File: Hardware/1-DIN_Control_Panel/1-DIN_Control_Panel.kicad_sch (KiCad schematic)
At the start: 82 parts, among them J1 Selector Knob Connector, J2 Rotary Switch 1x7, J3 2x05 Molex Micro-Fit 3.0 43045, J4 UART Expansion, J5 SW - Aux Jump-Start, J6 SW - Battery Bypass, J7 SW - Master Power, J8 Pot/SW - Brightness, K1 FINDER-40.52, U1 CA56-12SEKWA, U2 CA56-12SEKWA, U3 LTV-847S, U4 LTV-847S, U5 MAX 6954 - SSOP, U6 MAX 6954 - SSOP, U7 LM324DR, U8 12V->5V Variable Boost Buck C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

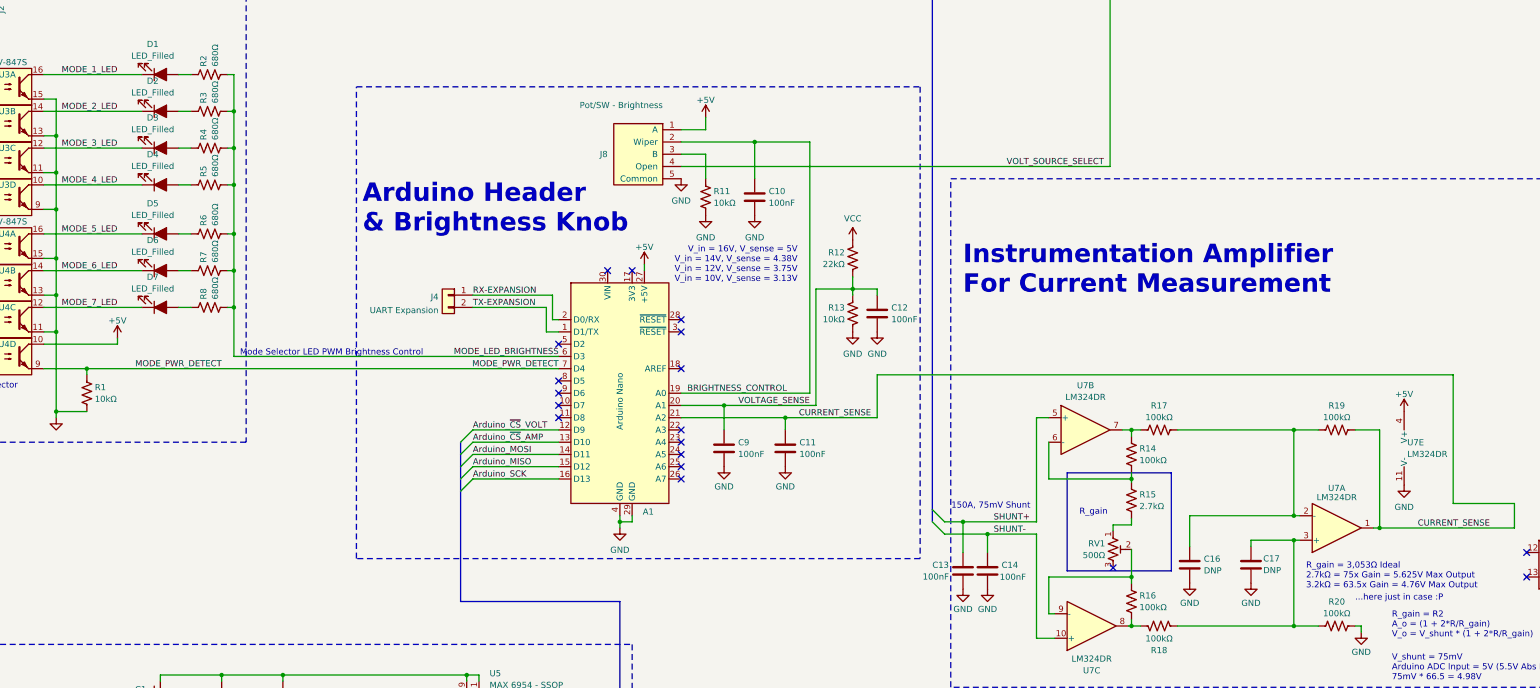
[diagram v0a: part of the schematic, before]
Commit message: Scooted some stuffs
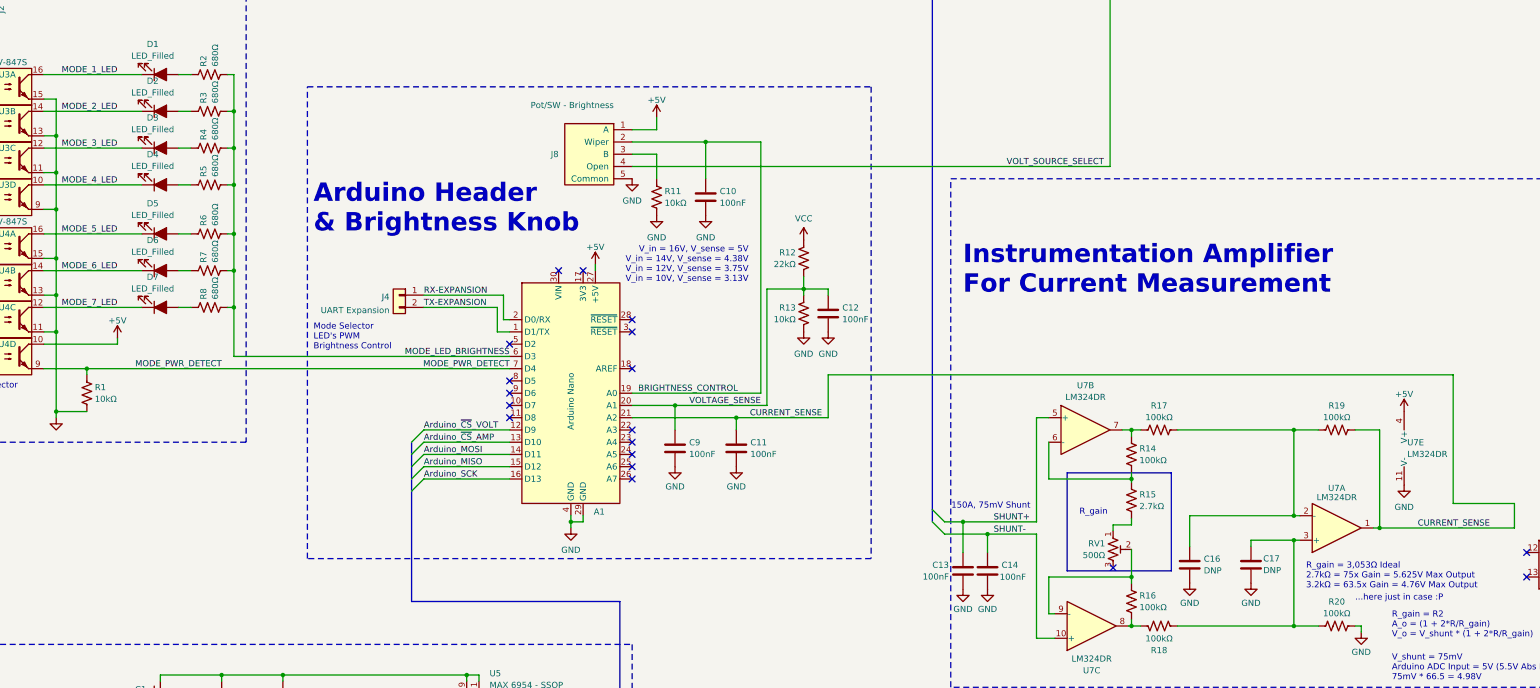
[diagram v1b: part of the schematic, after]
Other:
- note added: "Mode Selector LED's PWM Brightness Control"
- note removed: "Mode Selector LED PWM Brightness Control"
- moved on the sheet: A1, C10, C11, C12, C9, J4, J8, R11, R12, R13
